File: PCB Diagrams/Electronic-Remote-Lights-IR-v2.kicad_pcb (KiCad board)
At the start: 2 copper layers, 60.9 x 59.7 mm, 16 parts, among them J1 POWER, J2 220V, K1 RELAY, SW1 RESET, U1 VS1338B

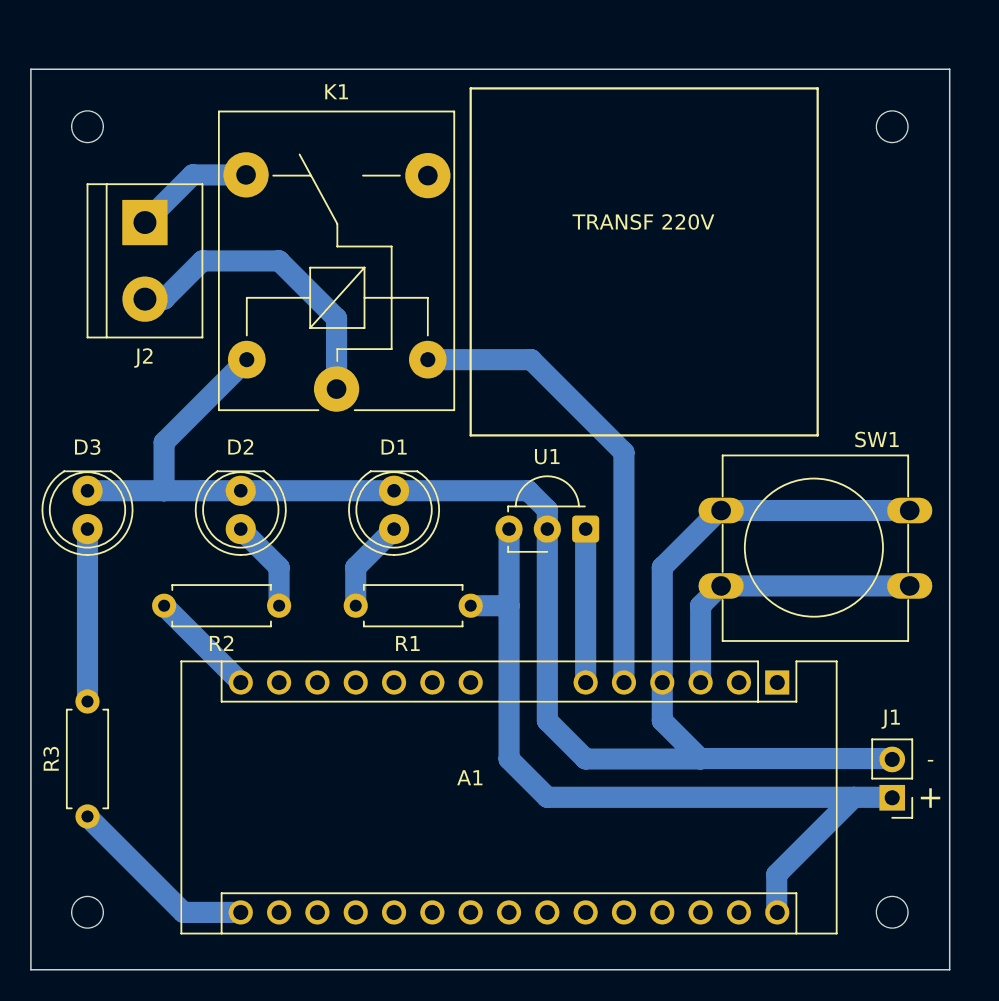
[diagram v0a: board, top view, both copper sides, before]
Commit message: PCB bug fix
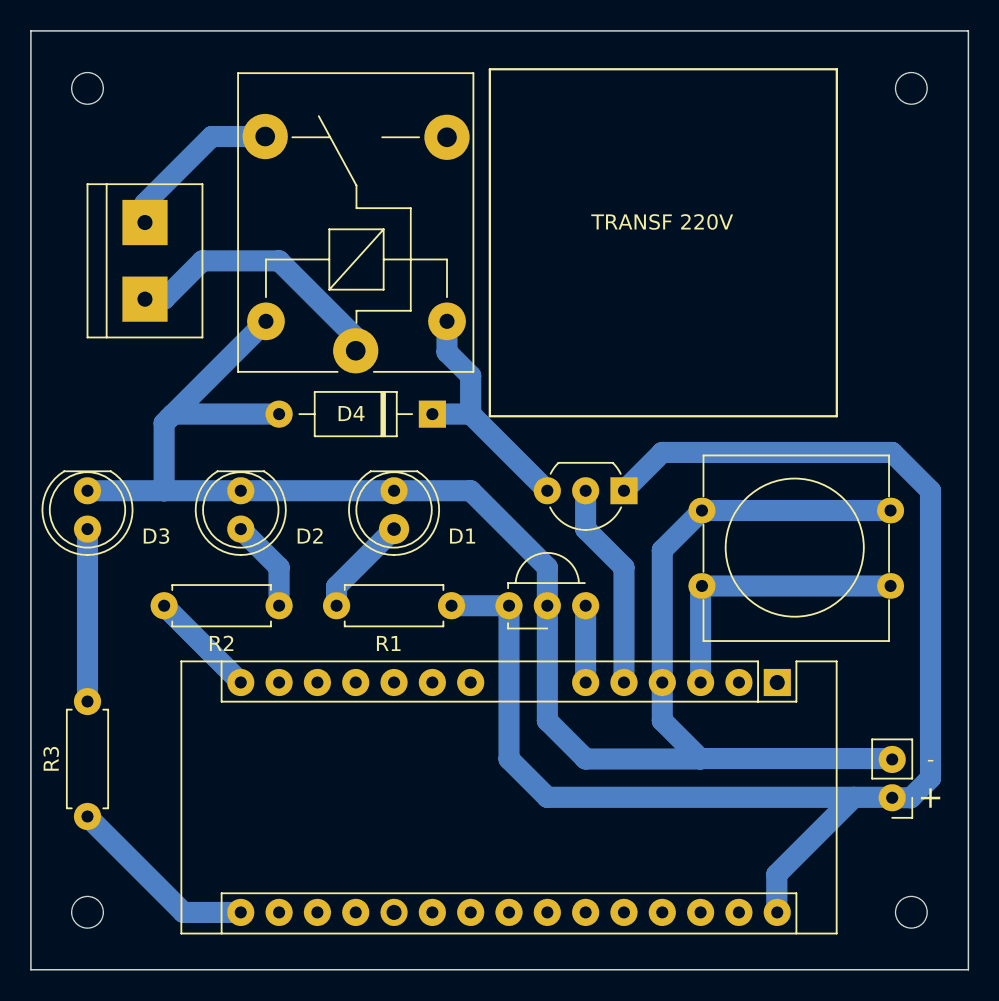
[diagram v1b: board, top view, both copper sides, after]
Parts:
- added D4: 1N4007, Diode_THT:D_DO-41_SOD81_P10.16mm_Horizontal, F.Cu at (101.6, 119.4)
- added Q1: BC547, Package_TO_SOT_THT:TO-92_Inline_Wide, F.Cu at (114.3, 124.5)
- moved U1 5.08 mm to (111.8, 132.1)
- moved K1 2.84 mm to (96.5, 115.2)
- moved H2 2.84 mm to (133.3, 97.8)
- moved H1 2.54 mm to (78.7, 97.8)
- moved SW1 1.27 mm to (132.0, 130.8)
- moved R1 1.27 mm to (102.9, 132.1)
- moved H3 1.27 mm to (133.3, 152.4)
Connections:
- K1 pad 2: Net-(A1-Pad5) -> Net-(K1-Pad2)
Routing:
- net +5V: track 54.0 -> 94.7 mm
- net Net-(A1-Pad5): track 30.8 -> 13.8 mm
- net Net-(K1-Pad2): track 0.00 -> 16.5 mm
- net GND: track 111.5 -> 119.3 mm
- net Net-(A1-Pad6): track 10.2 -> 5.09 mm
- net NEUT: track 8.01 -> 11.1 mm
- net LINE: track 20.0 -> 18.0 mm
- net Net-(D1-Pad2): track 6.13 -> 6.66 mm
- net Net-(A1-Pad3): track 19.5 -> 19.0 mm
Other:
- board size 60.9 x 59.7 mm -> 62.1 x 62.2 mm
